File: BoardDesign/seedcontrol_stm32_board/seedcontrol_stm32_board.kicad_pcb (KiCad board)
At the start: 2 copper layers, 90 x 72 mm, 50 parts, among them J1 Input, J2 Conn_01x02_Pin, U2 MP1584EN, U3 STM32F401RCTx

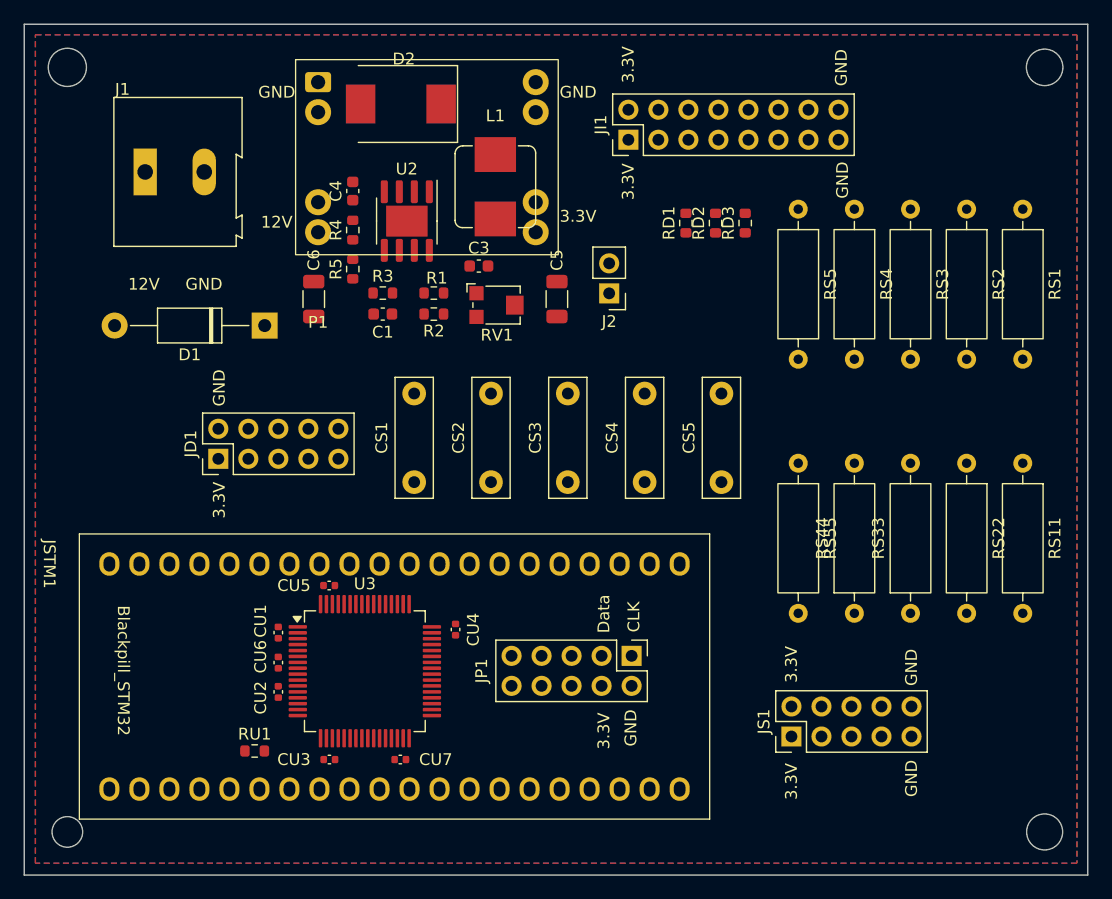
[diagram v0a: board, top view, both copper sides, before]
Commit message: Final Board design.
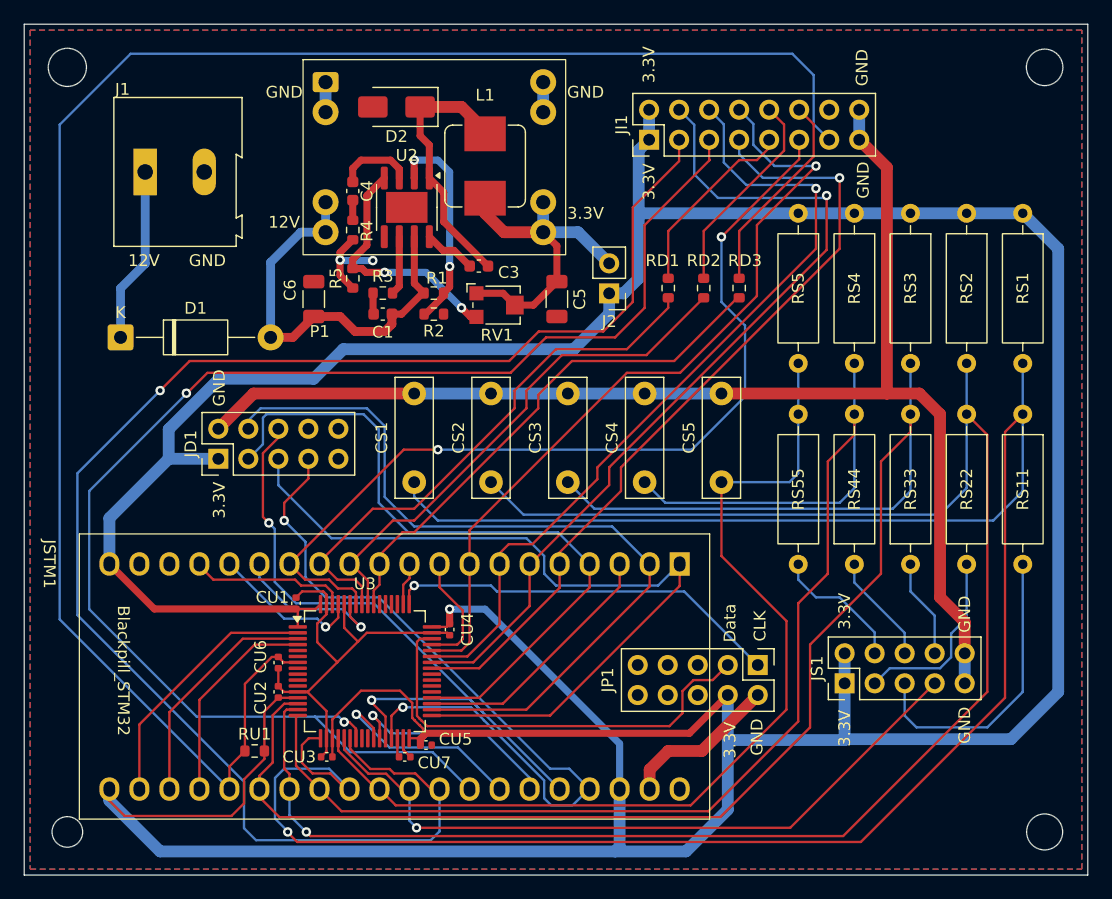
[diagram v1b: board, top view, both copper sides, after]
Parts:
- D2: footprint Diode_SMD:D_SMC -> Diode_SMD:D_SMA
- RS1, RS2, RS3, RS4, RS5: value 4,7k -> 4,7-10k
- RV1: value R_Potentiometer -> R_Pot
- moved CU5 15.8 mm to (109.0, 101.0)
- moved D1 12.2 mm to (83.2, 66.5), turned to 0 degrees
- moved JP1 10.7 mm to (137.1, 94.2)
- moved JS1 6.36 mm to (144.4, 95.8)
- moved RD1 5.70 mm to (129.5, 62.3), turned to -90 degrees
- moved RD2 5.59 mm to (132.5, 62.3)
- moved RD3 5.52 mm to (135.5, 62.3)
- moved RS11 4.15 mm to (159.5, 73.0)
- moved RS22 4.15 mm to (154.8, 73.0)
- moved RS55 4.15 mm to (140.5, 73.0)
- moved RS33 4.15 mm to (150.0, 85.7)
- moved RS44 4.15 mm to (145.2, 85.7)
- moved CU1 2.90 mm to (98.0, 89.0), turned to -90 degrees
- moved L1 1.95 mm to (114.0, 52.0)
- moved JI1 1.75 mm to (127.9, 49.8)
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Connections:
- net /3,3V renamed /V3,3
- C1 pad 2: Net-(D1-A) -> /V12
- C6 pad 2: +12V -> /V12
- D1 pad 1: Net-(D1-A) -> +12V
- D1 pad 2: +12V -> /V12
- P1 pad 3: +12V -> /V12
- P1 pad 4: +12V -> /V12
- R1 pad 2: Net-(D1-A) -> /V12
- U2 pad 7: Net-(D1-A) -> /V12
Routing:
- net +3.3V: track 0.00 -> 377.1 mm, vias 0 -> 1
- net GND: track 0.00 -> 179.5 mm, vias 0 -> 2
- net /PA3: track 0.00 -> 176.5 mm, vias 0 -> 1
- net /PA1: track 0.00 -> 152.1 mm, vias 0 -> 1
- net /RESET: track 0.00 -> 150.3 mm
- net /PA6: track 0.00 -> 135.0 mm, vias 0 -> 1
- net /PA0: track 0.00 -> 131.1 mm
- net /PA7: track 0.00 -> 123.6 mm, vias 0 -> 2
- net /PA2: track 0.00 -> 109.1 mm
- net /PA4: track 0.00 -> 82.4 mm
- net /PB6: track 0.00 -> 77.3 mm, vias 0 -> 2
- net /PA9: track 0.00 -> 73.5 mm, vias 0 -> 1
- net /PA10: track 0.00 -> 69.7 mm, vias 0 -> 1
- net /PB12: track 0.00 -> 68.7 mm
- net /PB13: track 0.00 -> 68.7 mm
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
